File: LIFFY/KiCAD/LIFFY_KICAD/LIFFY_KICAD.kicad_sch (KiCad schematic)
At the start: 13 parts, among them IC1 MC9S08MP16xLC, J1 VIN, J14 VIN2, J8 5V_OUT, Y1 Crystal 4 MHz

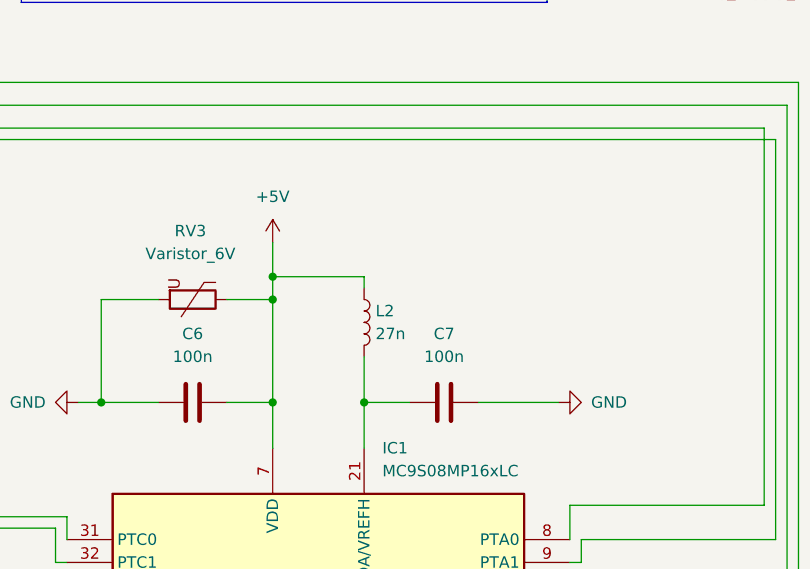
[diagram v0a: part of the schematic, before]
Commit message: V3 Fixed
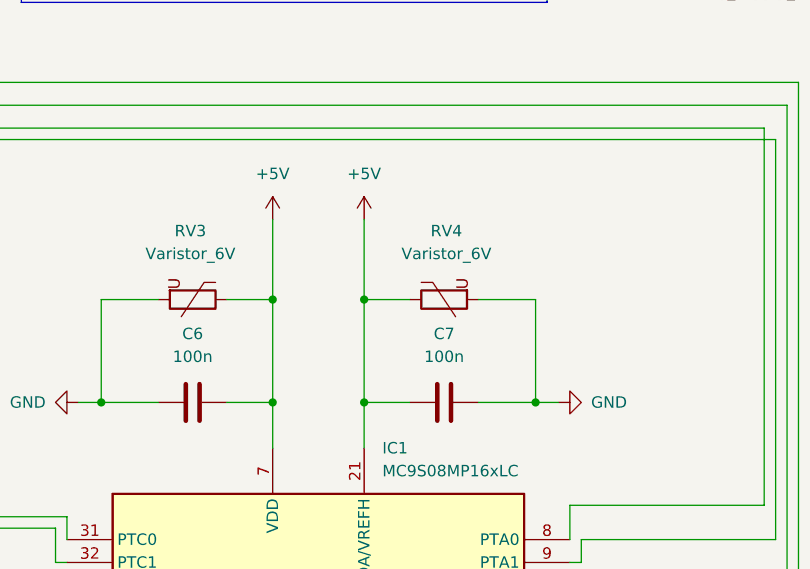
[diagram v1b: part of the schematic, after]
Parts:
- removed L2: 27n, Inductor_SMD:L_0805_2012Metric, symbol Device:L
- added RV4: Varistor_6V, Capacitor_SMD:C_0805_2012Metric, symbol Device:Varistor
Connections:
- net +5V: now also C7.2, IC1.21 (VDDA/VREFH), RV4.1
- net GND: now also RV4.2

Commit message: V2 PCB ADDED
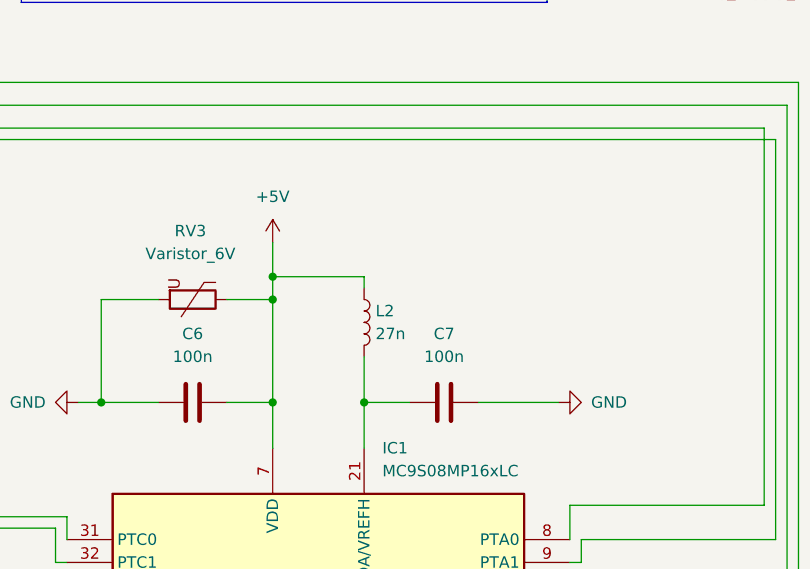
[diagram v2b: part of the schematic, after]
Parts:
- removed RV4: Varistor_6V, Capacitor_SMD:C_0805_2012Metric, symbol Device:Varistor
- added L2: 27n, Inductor_SMD:L_0805_2012Metric, symbol Device:L
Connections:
- net +5V: now also L2.1; no longer C7.2, IC1.21 (VDDA/VREFH)
- new net: C7.2, IC1.21 (VDDA/VREFH), L2.2
